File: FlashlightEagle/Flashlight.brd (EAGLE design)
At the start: 63.5 x 50.5 mm, 32 parts, among them IC1 7805T, IC2 TP4056, T1 BC547, T2 BC547, T3 BC547, X2 Filiament, X3 LED, X4 Switch, X5 Input

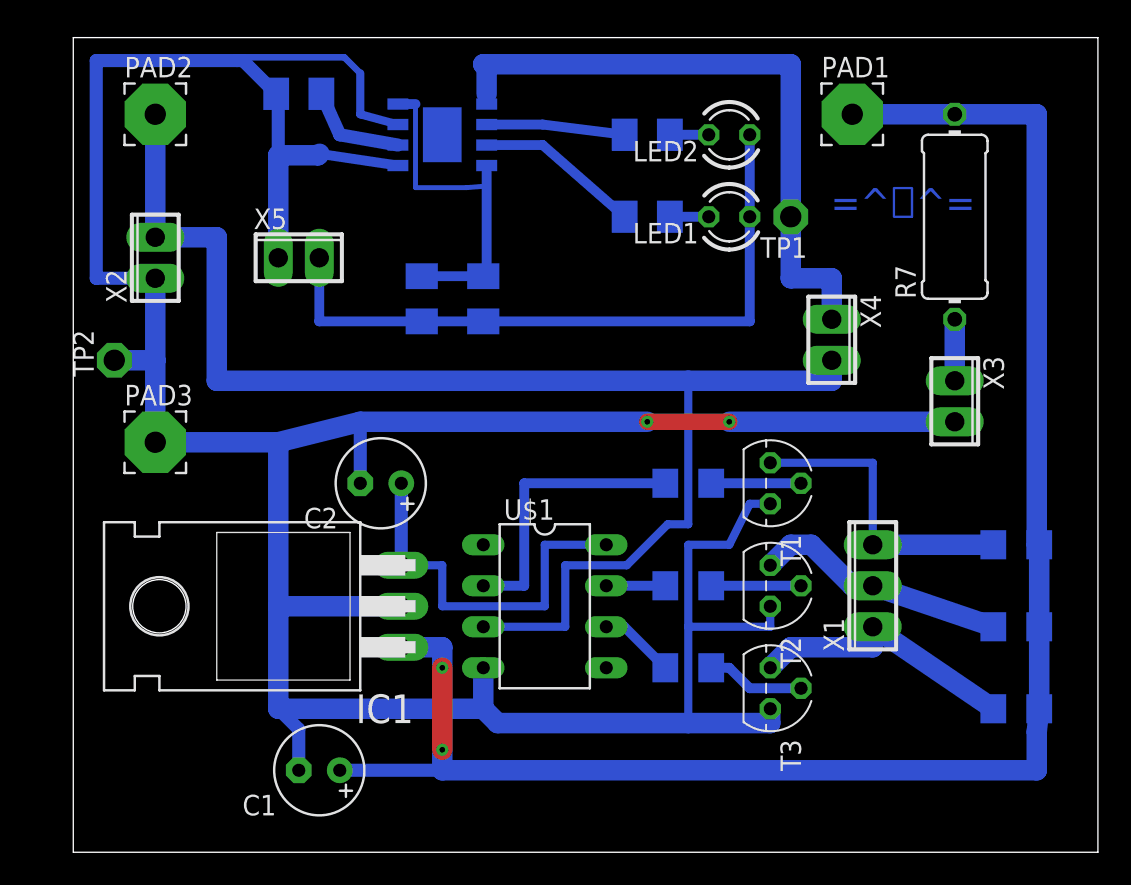
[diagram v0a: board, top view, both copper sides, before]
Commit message: Add files via upload
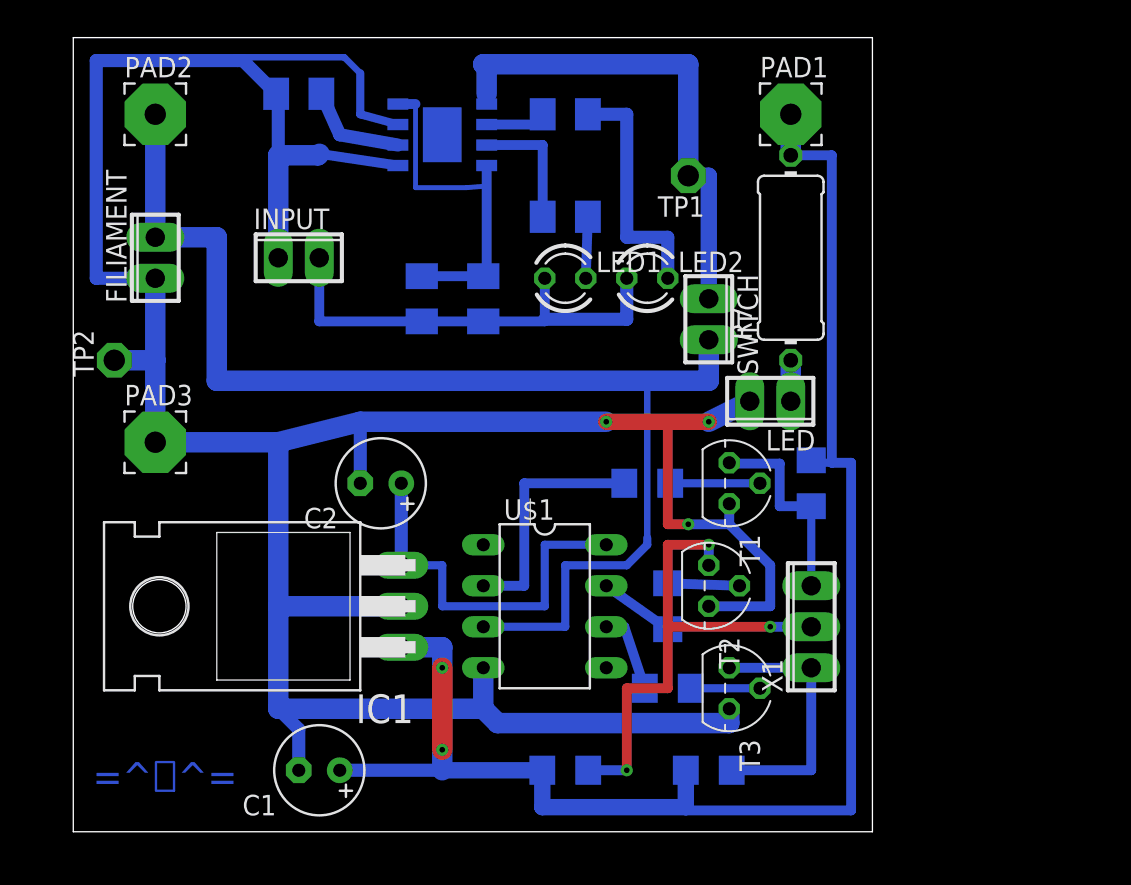
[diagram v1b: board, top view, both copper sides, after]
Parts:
- removed X3: LED, con-phoenix-254:2POL254
- removed X4: Switch, con-phoenix-254:2POL254
- added LED, SWITCH: (no value), con-phoenix-254:2POL254
- FILIAMENT: value Filiament -> (none)
- INPUT: value Input -> (none)
- moved R5 29.3 mm to (30.5, -1.27), turned to 180 degrees
- moved R6 19.4 mm to (39.4, -1.27), turned to 180 degrees
- moved R4 13.3 mm to (45.7, 16.5), turned to 90 degrees
- moved LED1 10.9 mm to (30.5, 29.2), turned to 0 degrees
- moved R7 10.5 mm to (44.5, 30.5)
- moved LED2 10.2 mm to (35.6, 29.2), turned to 0 degrees
- moved TP1 6.84 mm to (38.1, 35.6)
- moved R10 5.24 mm to (30.5, 39.4)
- moved R9 5.08 mm to (30.5, 33.0)
- moved X1 4.58 mm to (45.7, 7.62)
- moved T2 3.81 mm to (39.4, 10.2)
- moved PAD1 3.81 mm to (44.5, 39.4)
- moved R1 2.54 mm to (35.6, 16.5)
- moved T1 2.54 mm to (40.6, 16.5)
- moved T3 2.54 mm to (40.6, 3.81)
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- renumbered X2 to FILIAMENT, X5 to INPUT
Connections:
- net GND: now also LED.2; no longer X3.2
- net N$17: now also SWITCH.1; no longer X4.1
- net N$7: now also SWITCH.2; no longer X4.2
- net N$8: now also LED.1; no longer X3.1
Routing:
- net N$5: track 15.8 -> 31.6 mm, vias 0 -> 3
- net GND: track 214.1 -> 199.0 mm, vias 2 -> 3
- net N$22: track 42.2 -> 28.2 mm
- net N$21: track 2.41 -> 15.1 mm
- net N$17: track 39.9 -> 31.0 mm
- net VCC: track 105.6 -> 97.1 mm
- net N$4: track 18.9 -> 12.7 mm
- net N$14: track 8.59 -> 4.10 mm
- net N$7: track 86.1 -> 81.8 mm
- net N$12: track 17.6 -> 15.1 mm
- net N$9: track 10.2 -> 7.91 mm
- net N$3: track 6.09 -> 4.29 mm
- net N$20: track 2.41 -> 3.81 mm
- net N$8: track 3.81 -> 2.54 mm
- net N$2: track 5.56 -> 4.45 mm
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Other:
- board size 63.5 x 50.5 mm -> 49.5 x 49.2 mm

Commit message: Add files via upload
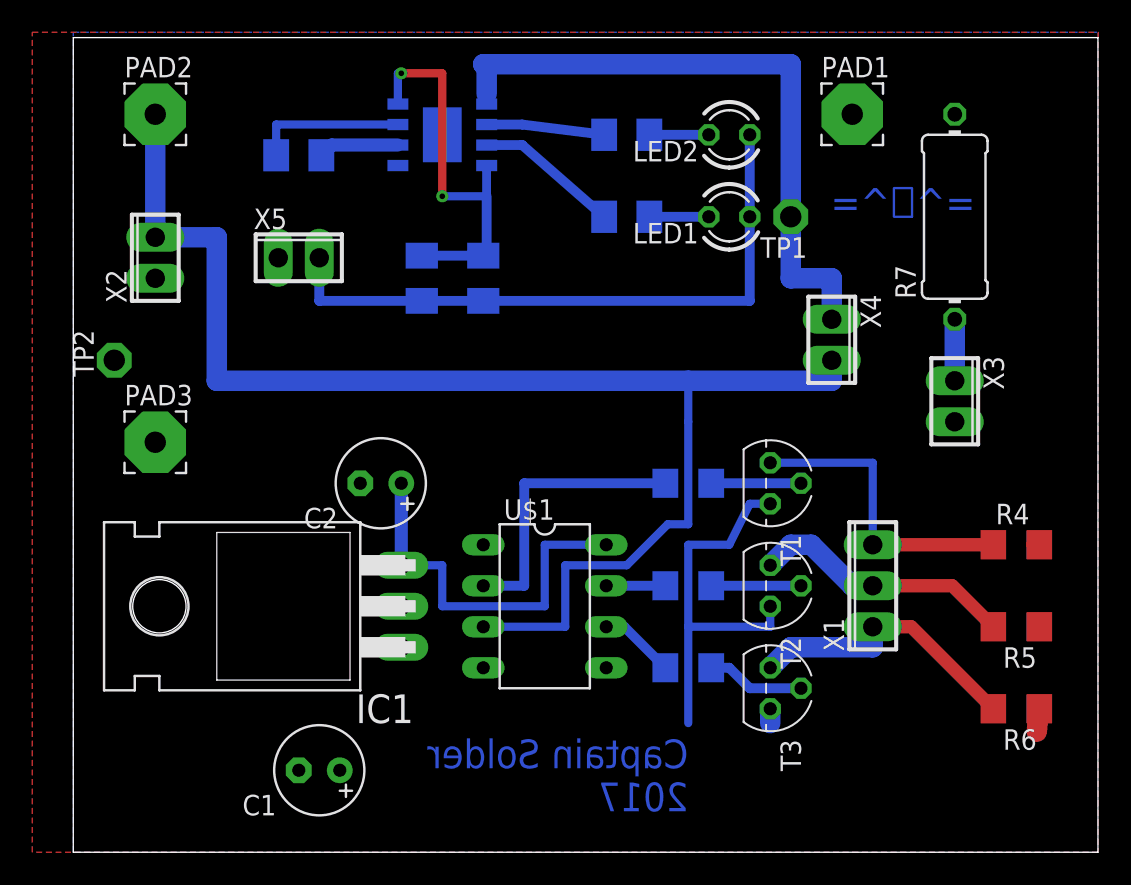
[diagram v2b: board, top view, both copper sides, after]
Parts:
- removed LED, SWITCH: (no value), con-phoenix-254:2POL254
- added X3: LED, con-phoenix-254:2POL254
- added X4: Switch, con-phoenix-254:2POL254
- X2: value (none) -> Filiament
- X5: value (none) -> Input
- moved R5 29.3 mm to (58.4, 7.62), flipped to the top
- moved R6 19.4 mm to (58.4, 2.54), flipped to the top
- moved R4 13.3 mm to (58.4, 12.7), flipped to the top, turned to 0 degrees
- moved LED1 10.9 mm to (40.6, 33.0), turned to 180 degrees
- moved R7 10.5 mm to (54.6, 33.0)
- moved LED2 10.2 mm to (40.6, 38.1), turned to 180 degrees
- moved TP1 6.84 mm to (44.5, 33.0)
- moved X1 4.58 mm to (49.5, 10.2)
- moved R10 4.02 mm to (34.3, 38.1)
- moved R8 3.81 mm to (14.0, 36.8)
- moved T2 3.81 mm to (43.2, 10.2)
- moved R9 3.81 mm to (34.3, 33.0)
- moved PAD1 3.81 mm to (48.3, 39.4)
- moved R1 2.54 mm to (38.1, 16.5)
- moved T1 2.54 mm to (43.2, 16.5)
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- renumbered FILIAMENT to X2, INPUT to X5
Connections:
- net GND: now also X3.2; no longer LED.2
- net N$17: now also X4.1; no longer SWITCH.1
- net N$7: now also X4.2; no longer SWITCH.2
- net N$8: now also X3.1; no longer LED.1
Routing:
- net GND: track 199.0 -> 34.8 mm, vias 3 -> 0
- net VCC: track 97.1 -> 2.85 mm, vias 2 -> 0
- net N$5: track 31.6 -> 16.4 mm, vias 3 -> 0
- net N$21: track 15.1 -> 3.68 mm
- net N$22: track 28.2 -> 39.6 mm
- net N$17: track 31.0 -> 39.9 mm
- net N$4: track 12.7 -> 18.9 mm
- net N$16: track 22.9 -> 27.8 mm, vias 0 -> 2
- net N$7: track 81.8 -> 86.1 mm
- net N$14: track 4.10 -> 7.32 mm
- net N$12: track 15.1 -> 17.6 mm
- net N$3: track 4.29 -> 6.09 mm
- net N$15: track 6.44 -> 5.00 mm
- net N$6: track 16.4 -> 17.7 mm
- net N$8: track 2.54 -> 3.81 mm
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- added copper zone on layer 16, net GND
- added copper zone on layer 1, net VCC
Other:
- board size 49.5 x 49.2 mm -> 63.5 x 50.5 mm
- board text added: "Captain Solder 2017"
